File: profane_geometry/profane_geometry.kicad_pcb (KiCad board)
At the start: 4 copper layers, 71.1 x 53.3 mm, 105 parts, among them J1 Conn_01x12, J2 Conn_01x12, Q1 MMBF4416A, U1 LM1117-3.3, U2 TL074, U3 TL074, U4 TL074, U5 TL074, U6 TL072, U7 MCP6002-xSN, U8 MCP4728

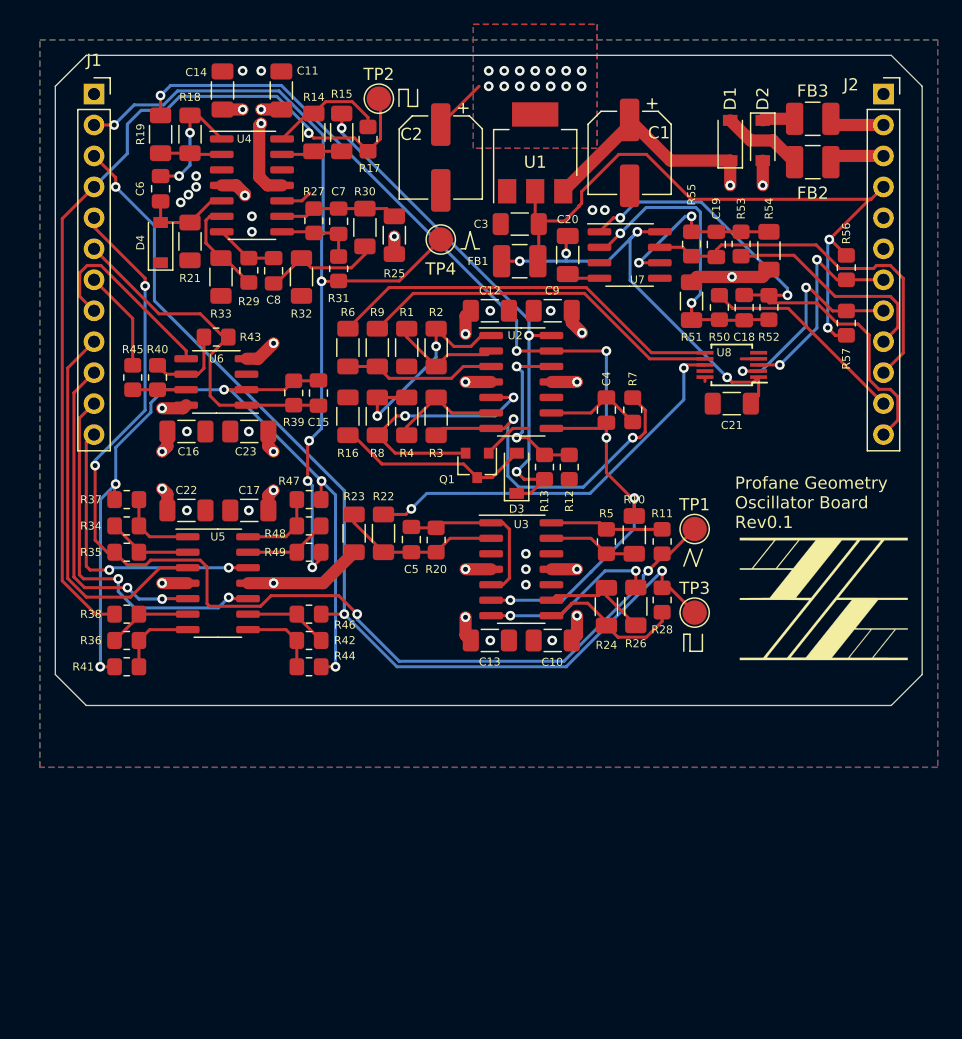
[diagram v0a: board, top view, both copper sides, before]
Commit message: update .gitignore, current kicad project
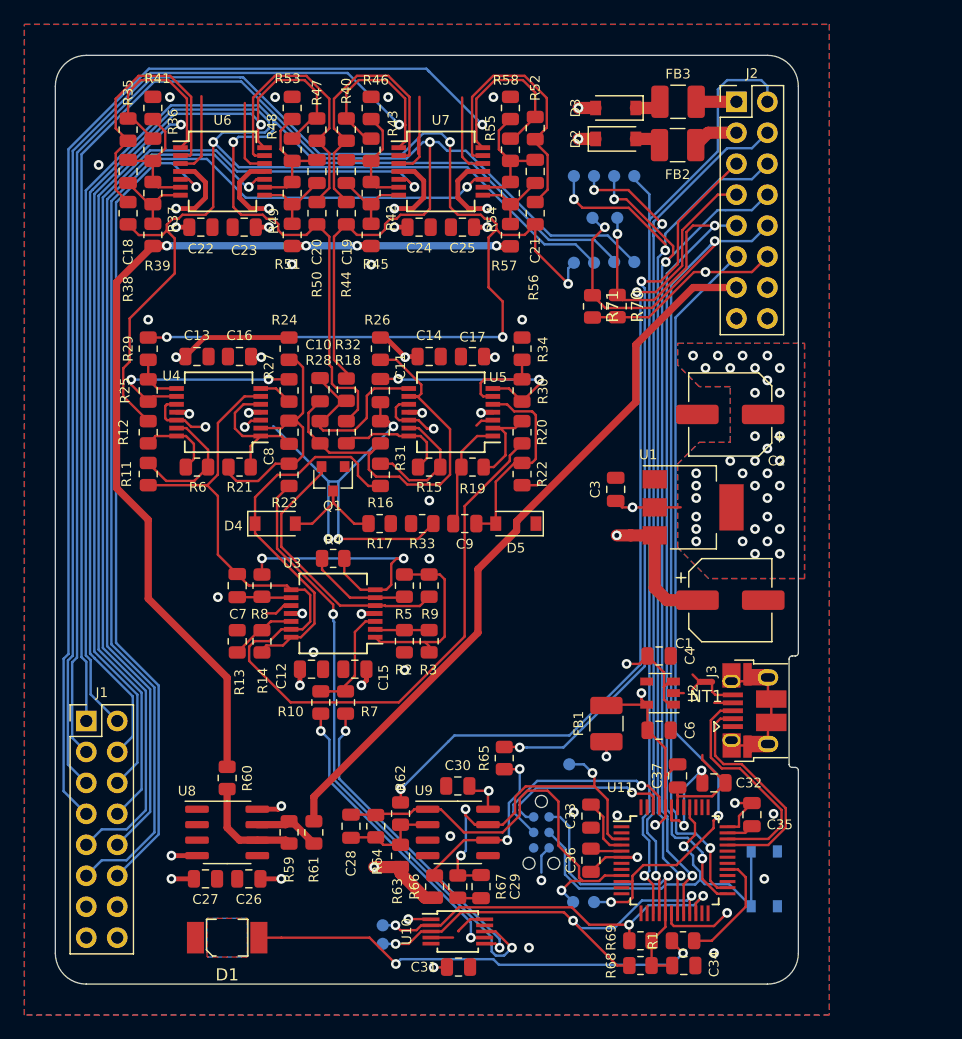
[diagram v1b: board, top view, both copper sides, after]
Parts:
- removed C5: 2.2nF, Capacitor_SMD:C_0805_2012Metric_Pad1.18x1.45mm_HandSolder
- removed REF**: OSHW-Symbol_6.7x6mm_SilkScreen, profane_geometry:OSHW-Symbol_6.7x6mm_SilkScreen
- removed Ref**: Val**, profane_geometry:zzzzzzzz_back_soldermask
- removed Ref**: Val**, profane_geometry:zzzzzzzz_new_front_soldermask
- added C24: 0.1uF, Capacitor_SMD:C_0805_2012Metric, F.Cu at (146.7, 59.8)
- added C25: 0.1uF, Capacitor_SMD:C_0805_2012Metric, F.Cu at (150.2, 59.8)
- added C26: 0.1uF, Capacitor_SMD:C_0805_2012Metric, F.Cu at (132.7, 113.3)
- added C27: 0.1uF, Capacitor_SMD:C_0805_2012Metric, F.Cu at (129.2, 113.3)
- added C28: 4.7nF, Capacitor_SMD:C_0805_2012Metric, F.Cu at (141.1, 109.0)
- added C29: 2.2nF, Capacitor_SMD:C_0805_2012Metric, F.Cu at (151.8, 113.9)
- added C30: 0.1uF, Capacitor_SMD:C_0805_2012Metric, F.Cu at (149.9, 105.7)
- added C31: 0.1uF, Capacitor_SMD:C_0805_2012Metric, F.Cu at (149.9, 120.5)
- added C32: 1uF, Capacitor_SMD:C_0805_2012Metric, F.Cu at (170.9, 105.4)
- added C33: 0.1uF, Capacitor_SMD:C_0805_2012Metric, F.Cu at (160.8, 108.1)
- added C34: 0.1uF, Capacitor_SMD:C_0805_2012Metric, F.Cu at (168.4, 120.4)
- added C35: 0.1uF, Capacitor_SMD:C_0805_2012Metric, F.Cu at (174.0, 108.0)
- added C36: 0.1uF, Capacitor_SMD:C_0805_2012Metric, F.Cu at (160.8, 111.8)
- added C37: 0.1uF, Capacitor_SMD:C_0805_2012Metric, F.Cu at (167.9, 104.8)
- added D5: 1N5819, Diode_SMD:D_SOD-123, F.Cu at (154.6, 84.1)
- added J3: USB_B_Micro, Connector_USB:USB_Micro-B_Amphenol_10103594-0001LF_Horizontal, F.Cu at (174.2, 99.5)
- added J4: TagConect SWD, Connector:Tag-Connect_TC2030-IDC-NL_2x03_P1.27mm_Vertical, B.Cu at (156.7, 109.5)
- added NT1: GND_Net_Tie, NetTie:NetTie-2_SMD_Pad0.5mm, F.Cu at (170.2, 97.1)
- added R58: 22k, Resistor_SMD:R_0805_2012Metric, F.Cu at (154.2, 50.0)
- added R59: 10k, Resistor_SMD:R_0805_2012Metric, F.Cu at (136.0, 109.5)
- added R60: 10k, Resistor_SMD:R_0805_2012Metric, F.Cu at (130.9, 105.0)
- added R61: 1k, Resistor_SMD:R_0805_2012Metric, F.Cu at (138.0, 109.5)
- added R62: 100k, Resistor_SMD:R_0805_2012Metric, F.Cu at (145.2, 107.9)
- added R63: 240k, Resistor_SMD:R_0805_2012Metric, F.Cu at (145.2, 111.4)
- added R64: 64.9k, Resistor_SMD:R_0805_2012Metric, F.Cu at (143.1, 109.0)
- added R65: 100k, Resistor_SMD:R_0805_2012Metric, F.Cu at (153.7, 103.4)
- added R66: 240k, Resistor_SMD:R_0805_2012Metric, F.Cu at (148.0, 113.9)
- added R67: 56k, Resistor_SMD:R_0805_2012Metric, F.Cu at (149.9, 113.9)
- added R68: 4.7k, Resistor_SMD:R_0805_2012Metric, F.Cu at (164.8, 120.4)
- added R69: 4.7k, Resistor_SMD:R_0805_2012Metric, F.Cu at (164.8, 118.4)
- added R70: 4.7k, Resistor_SMD:R_0805_2012Metric, F.Cu at (162.9, 66.3)
- added R71: 4.7k, Resistor_SMD:R_0805_2012Metric, F.Cu at (160.9, 66.3)
- added SW1: RESET_SW, zzzzzzzz:SPST_TL3365AF180QG_SMD, B.Cu at (175.0, 113.3)
- added TP10: PSL, TestPoint:TestPoint_Pad_D1.0mm, B.Cu at (159.4, 55.6)
- added TP11: NSL, TestPoint:TestPoint_Pad_D1.0mm, B.Cu at (162.7, 55.6)
- added TP12: D_SDA, TestPoint:TestPoint_Pad_D1.0mm, B.Cu at (143.7, 118.6)
- added TP13: D_SCL, TestPoint:TestPoint_Pad_D1.0mm, B.Cu at (143.7, 117.1)
- added TP14: L_SDA, TestPoint:TestPoint_Pad_D1.0mm, B.Cu at (162.9, 59.1)
- added TP15: L_SCL, TestPoint:TestPoint_Pad_D1.0mm, B.Cu at (160.9, 59.1)
- added TP5: V/OCT, TestPoint:TestPoint_Pad_D1.0mm, B.Cu at (159.0, 103.9)
- added TP6: PWM, TestPoint:TestPoint_Pad_D1.0mm, B.Cu at (159.3, 115.2)
- added TP7: POT, TestPoint:TestPoint_Pad_D1.0mm, B.Cu at (161.0, 115.2)
- added TP8: TSL, TestPoint:TestPoint_Pad_D1.0mm, B.Cu at (164.3, 55.6)
- added TP9: SSL, TestPoint:TestPoint_Pad_D1.0mm, B.Cu at (161.0, 55.6)
- added U10: MCP4728, Package_SO:MSOP-10_3x3mm_P0.5mm, F.Cu at (149.9, 117.6)
- added U11: ATSAMD21G18A-AUT, Package_QFP:TQFP-48_7x7mm_P0.5mm, F.Cu at (167.6, 111.8)
- added U9: MCP6002-xSN, Package_SO:SOIC-8_3.9x4.9mm_P1.27mm, F.Cu at (149.9, 109.5)
- C10: value 0.1uF -> 22pF; footprint Capacitor_SMD:C_1206_3216Metric_Pad1.33x1.80mm_HandSolder -> Capacitor_SMD:C_0805_2012Metric
- C11: value 0.1uF -> 4.7uF; footprint Capacitor_SMD:C_1206_3216Metric_Pad1.33x1.80mm_HandSolder -> Capacitor_SMD:C_0805_2012Metric
- C12, C13, C14, C16, C17, C22, C23, C3: footprint Capacitor_SMD:C_1206_3216Metric_Pad1.33x1.80mm_HandSolder -> Capacitor_SMD:C_0805_2012Metric
- C15: value 8.2pF -> 0.1uF; footprint Capacitor_SMD:C_0805_2012Metric_Pad1.18x1.45mm_HandSolder -> Capacitor_SMD:C_0805_2012Metric
- C18: value 4.7nF -> 47pF; footprint Capacitor_SMD:C_0805_2012Metric_Pad1.18x1.45mm_HandSolder -> Capacitor_SMD:C_0805_2012Metric
- C19: value 2.2nF -> 47pF; footprint Capacitor_SMD:C_0805_2012Metric_Pad1.18x1.45mm_HandSolder -> Capacitor_SMD:C_0805_2012Metric
- C20, C21: value 0.1uF -> 47pF; footprint Capacitor_SMD:C_1206_3216Metric_Pad1.33x1.80mm_HandSolder -> Capacitor_SMD:C_0805_2012Metric
- C4: value 47nF -> 1uF; footprint Capacitor_SMD:C_0805_2012Metric_Pad1.18x1.45mm_HandSolder -> Capacitor_SMD:C_0805_2012Metric
- C6: value 10uF -> 1uF; footprint Capacitor_SMD:C_0805_2012Metric_Pad1.18x1.45mm_HandSolder -> Capacitor_SMD:C_0805_2012Metric
- C7: value 22pF -> 47nF; footprint Capacitor_SMD:C_0805_2012Metric_Pad1.18x1.45mm_HandSolder -> Capacitor_SMD:C_0805_2012Metric
- C8: value 10uF -> 2.2nF; footprint Capacitor_SMD:C_0805_2012Metric_Pad1.18x1.45mm_HandSolder -> Capacitor_SMD:C_0805_2012Metric
- C9: value 0.1uF -> 1uF; footprint Capacitor_SMD:C_1206_3216Metric_Pad1.33x1.80mm_HandSolder -> Capacitor_SMD:C_0805_2012Metric
- D1: value 1N5819 -> PWR; footprint Diode_SMD:D_SOD-123 -> zzzzzzzz:SunLED-Rev-2-PLCC-SeeThru
- J1, J2: value Conn_01x12 -> Conn_02x08_Odd_Even; footprint Connector_PinSocket_2.54mm:PinSocket_1x12_P2.54mm_Vertical -> Connector_PinHeader_2.54mm:PinHeader_2x08_P2.54mm_Vertical
- R1: value 10k -> 330R; footprint Resistor_SMD:R_1206_3216Metric_Pad1.30x1.75mm_HandSolder -> Resistor_SMD:R_0805_2012Metric
- R10: value 10k -> 1M; footprint Resistor_SMD:R_1206_3216Metric_Pad1.30x1.75mm_HandSolder -> Resistor_SMD:R_0805_2012Metric
- R11, R17, R31, R45, R7: value 1k -> 10k; footprint Resistor_SMD:R_0805_2012Metric_Pad1.20x1.40mm_HandSolder -> Resistor_SMD:R_0805_2012Metric
- R12: value 7.15k -> 1k; footprint Resistor_SMD:R_0805_2012Metric_Pad1.20x1.40mm_HandSolder -> Resistor_SMD:R_0805_2012Metric
- R13: value 2.87k -> 7.15k; footprint Resistor_SMD:R_0805_2012Metric_Pad1.20x1.40mm_HandSolder -> Resistor_SMD:R_0805_2012Metric
- R14: value 4.12k -> 2.87k; footprint Resistor_SMD:R_1206_3216Metric_Pad1.30x1.75mm_HandSolder -> Resistor_SMD:R_0805_2012Metric
- R15: value 10k -> 4.12k; footprint Resistor_SMD:R_1206_3216Metric_Pad1.30x1.75mm_HandSolder -> Resistor_SMD:R_0805_2012Metric
- R16, R2, R3, R4: footprint Resistor_SMD:R_1206_3216Metric_Pad1.30x1.75mm_HandSolder -> Resistor_SMD:R_0805_2012Metric
- R18: value 3.57k -> 1k; footprint Resistor_SMD:R_1206_3216Metric_Pad1.30x1.75mm_HandSolder -> Resistor_SMD:R_0805_2012Metric
- R19: value 10k -> 3.57k; footprint Resistor_SMD:R_1206_3216Metric_Pad1.30x1.75mm_HandSolder -> Resistor_SMD:R_0805_2012Metric
- R20: value 169k -> 10k; footprint Resistor_SMD:R_0805_2012Metric_Pad1.20x1.40mm_HandSolder -> Resistor_SMD:R_0805_2012Metric
- R21: value 47k -> 169k; footprint Resistor_SMD:R_1206_3216Metric_Pad1.30x1.75mm_HandSolder -> Resistor_SMD:R_0805_2012Metric
- R22: value 33k -> 47k; footprint Resistor_SMD:R_1206_3216Metric_Pad1.30x1.75mm_HandSolder -> Resistor_SMD:R_0805_2012Metric
- R23: value 240k -> 49.9k; footprint Resistor_SMD:R_1206_3216Metric_Pad1.30x1.75mm_HandSolder -> Resistor_SMD:R_0805_2012Metric
- R24: value 10k -> 240k; footprint Resistor_SMD:R_1206_3216Metric_Pad1.30x1.75mm_HandSolder -> Resistor_SMD:R_0805_2012Metric
- R25: value 47k -> 10k; footprint Resistor_SMD:R_1206_3216Metric_Pad1.30x1.75mm_HandSolder -> Resistor_SMD:R_0805_2012Metric
- R26: value 22k -> 47k; footprint Resistor_SMD:R_1206_3216Metric_Pad1.30x1.75mm_HandSolder -> Resistor_SMD:R_0805_2012Metric
- R27: value 8.25k -> 22k; footprint Resistor_SMD:R_0805_2012Metric_Pad1.20x1.40mm_HandSolder -> Resistor_SMD:R_0805_2012Metric
- R28: value 1k -> 8.25k; footprint Resistor_SMD:R_0805_2012Metric_Pad1.20x1.40mm_HandSolder -> Resistor_SMD:R_0805_2012Metric
- R29: value 30.1k -> 1k; footprint Resistor_SMD:R_0805_2012Metric_Pad1.20x1.40mm_HandSolder -> Resistor_SMD:R_0805_2012Metric
- R30: value 10k -> 30.1k; footprint Resistor_SMD:R_1206_3216Metric_Pad1.30x1.75mm_HandSolder -> Resistor_SMD:R_0805_2012Metric
- R32: value 47k -> 1k; footprint Resistor_SMD:R_1206_3216Metric_Pad1.30x1.75mm_HandSolder -> Resistor_SMD:R_0805_2012Metric
- R33: value 10k -> 100k; footprint Resistor_SMD:R_1206_3216Metric_Pad1.30x1.75mm_HandSolder -> Resistor_SMD:R_0805_2012Metric
- R34, R35, R40: value 20k -> 10k; footprint Resistor_SMD:R_0805_2012Metric_Pad1.20x1.40mm_HandSolder -> Resistor_SMD:R_0805_2012Metric
- R36, R43, R48: value 20k -> 2.2M; footprint Resistor_SMD:R_0805_2012Metric_Pad1.20x1.40mm_HandSolder -> Resistor_SMD:R_0805_2012Metric
- R37: value 100k -> 47k; footprint Resistor_SMD:R_0805_2012Metric_Pad1.20x1.40mm_HandSolder -> Resistor_SMD:R_0805_2012Metric
- R38: value 20k -> 30.1k; footprint Resistor_SMD:R_0805_2012Metric_Pad1.20x1.40mm_HandSolder -> Resistor_SMD:R_0805_2012Metric
- R39, R47: value 100k -> 10k; footprint Resistor_SMD:R_0805_2012Metric_Pad1.20x1.40mm_HandSolder -> Resistor_SMD:R_0805_2012Metric
- R41, R53: value 100k -> 22k; footprint Resistor_SMD:R_0805_2012Metric_Pad1.20x1.40mm_HandSolder -> Resistor_SMD:R_0805_2012Metric
- R42, R49: value 20k -> 47k; footprint Resistor_SMD:R_0805_2012Metric_Pad1.20x1.40mm_HandSolder -> Resistor_SMD:R_0805_2012Metric
- R44, R50: value 100k -> 30.1k; footprint Resistor_SMD:R_0805_2012Metric_Pad1.20x1.40mm_HandSolder -> Resistor_SMD:R_0805_2012Metric
- R46: value 20k -> 22k; footprint Resistor_SMD:R_0805_2012Metric_Pad1.20x1.40mm_HandSolder -> Resistor_SMD:R_0805_2012Metric
- R5: value 5.9k -> 10k; footprint Resistor_SMD:R_0805_2012Metric_Pad1.20x1.40mm_HandSolder -> Resistor_SMD:R_0805_2012Metric
- R51: value 240k -> 10k; footprint Resistor_SMD:R_1206_3216Metric_Pad1.30x1.75mm_HandSolder -> Resistor_SMD:R_0805_2012Metric
- R52: value 64.9k -> 10k; footprint Resistor_SMD:R_0805_2012Metric_Pad1.20x1.40mm_HandSolder -> Resistor_SMD:R_0805_2012Metric
- R54: value 240k -> 47k; footprint Resistor_SMD:R_1206_3216Metric_Pad1.30x1.75mm_HandSolder -> Resistor_SMD:R_0805_2012Metric
- R55: value 56k -> 2.2M; footprint Resistor_SMD:R_0805_2012Metric_Pad1.20x1.40mm_HandSolder -> Resistor_SMD:R_0805_2012Metric
- R56: value 4.7k -> 30.1k; footprint Resistor_SMD:R_0805_2012Metric_Pad1.20x1.40mm_HandSolder -> Resistor_SMD:R_0805_2012Metric
- R57: value 4.7k -> 10k; footprint Resistor_SMD:R_0805_2012Metric_Pad1.20x1.40mm_HandSolder -> Resistor_SMD:R_0805_2012Metric
- R6: value 10k -> 5.6k; footprint Resistor_SMD:R_1206_3216Metric_Pad1.30x1.75mm_HandSolder -> Resistor_SMD:R_0805_2012Metric
- R8: value 10k -> 1k; footprint Resistor_SMD:R_1206_3216Metric_Pad1.30x1.75mm_HandSolder -> Resistor_SMD:R_0805_2012Metric
- R9: value 1M -> 10k; footprint Resistor_SMD:R_1206_3216Metric_Pad1.30x1.75mm_HandSolder -> Resistor_SMD:R_0805_2012Metric
- TP1, TP2, TP3, TP4: footprint TestPoint:TestPoint_Pad_D2.0mm -> TestPoint:TestPoint_Pad_D1.0mm; moved to B.Cu
- U1: value LM1117-3.3 -> LM1117-5
- U2: value TL074 -> AP2112K-3.3; footprint Package_SO:SOIC-14_3.9x8.7mm_P1.27mm -> Package_TO_SOT_SMD:SOT-23-5
- U3, U4, U5: footprint Package_SO:SOIC-14_3.9x8.7mm_P1.27mm -> Package_SO:SSOP-14_5.3x6.2mm_P0.65mm
- U6: value TL072 -> TL074; footprint Package_SO:SOIC-8_3.9x4.9mm_P1.27mm -> Package_SO:SSOP-14_5.3x6.2mm_P0.65mm
- U7: value MCP6002-xSN -> TL074; footprint Package_SO:SOIC-8_3.9x4.9mm_P1.27mm -> Package_SO:SSOP-14_5.3x6.2mm_P0.65mm
- U8: value MCP4728 -> TL072; footprint Package_SO:MSOP-10_3x3mm_P0.5mm -> Package_SO:SOIC-8_3.9x4.9mm_P1.27mm
- moved D1 77.3 mm to (130.9, 118.1), turned to 0 degrees
- moved C6 60.4 mm to (166.4, 101.1), turned to 0 degrees
- moved U8 56.4 mm to (130.9, 109.5), turned to 0 degrees
- moved R1 53.7 mm to (168.3, 118.4), turned to 180 degrees
- moved C18 51.8 mm to (122.8, 55.2), turned to 90 degrees
- moved J1 51.4 mm to (119.4, 100.3)
- moved R41 45.9 mm to (124.8, 50.0), turned to 270 degrees
- moved R11 42.5 mm to (124.5, 80.1), turned to 270 degrees
- moved R14 42.0 mm to (133.8, 93.8), turned to 90 degrees
- moved R46 41.8 mm to (142.7, 50.0), turned to 270 degrees
- moved R36 40.3 mm to (124.8, 53.5), turned to 90 degrees
- moved FB1 38.6 mm to (162.1, 100.5), turned to 90 degrees
- moved R53 38.5 mm to (136.3, 50.0)
- moved C1 37.6 mm to (172.2, 90.4), turned to 0 degrees
- moved R19 37.4 mm to (151.1, 79.5), turned to 0 degrees
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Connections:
- C10 pad 1: GND -> Net-(C10-Pad1)
- C10 pad 2: -12V -> Net-(C10-Pad2)
- C11 pad 1: GND -> Net-(C11-Pad1)
- C11 pad 2: -12V -> Net-(C11-Pad2)
- C12 pad 1: +12V -> GND
- C12 pad 2: GND -> -12V
- C13 pad 1: +12V -> GND
- C13 pad 2: GND -> -12V
- C14 pad 1: +12V -> GND
- C14 pad 2: GND -> -12V
- C15 pad 1: /mix-pre -> +12V
- C15 pad 2: Net-(C15-Pad2) -> GND
- C17 pad 1: GND -> +12V
- C17 pad 2: -12V -> GND
- C18 pad 1: /pulse-scaled -> Net-(C18-Pad1)
- C19 pad 1: /v_oct-scaled -> Net-(C19-Pad1)
- C2 pad 1: +3V3 -> +5V
- C20 pad 1: GND -> Net-(C20-Pad1)
- C20 pad 2: +3.3VA -> Net-(C20-Pad2)
- C21 pad 1: GND -> Net-(C21-Pad1)
- C21 pad 2: +3.3VA -> Net-(C21-Pad2)
- C3 pad 1: +3V3 -> +5V
- C4 pad 1: /Geometry Core/tri-pre -> +5V
- C4 pad 2: Net-(C4-Pad2) -> GND
- C6 pad 1: Net-(C6-Pad1) -> +3V3
- C6 pad 2: Net-(C6-Pad2) -> GND
- C7 pad 1: Net-(C7-Pad1) -> /Geometry Core/tri-pre
- C9 pad 1: GND -> Net-(C9-Pad1)
- C9 pad 2: -12V -> Net-(C9-Pad2)
- D1 pad 1: +12V -> GND
- D2 pad 1: Net-(D2-Pad1) -> +12V
- D2 pad 2: -12V -> Net-(D2-Pad2)
- D3 pad 1: /Geometry Core/square-pre -> Net-(D3-Pad1)
- D3 pad 2: Net-(D3-Pad2) -> -12V
- D4 pad 1: GND -> /Geometry Core/square-pre
- D4 pad 2: Net-(C6-Pad1) -> Net-(D4-Pad2)
- FB2 pad 1: Net-(D1-Pad2) -> Net-(D2-Pad2)
- FB3 pad 1: Net-(D2-Pad1) -> Net-(D3-Pad1)
- J1 pad 1: GND -> /notch-out
- J1 pad 10: /square-att-in -> /square-mix-in
- J1 pad 11: /pulse-att-in -> /pulse-mix-in
- J1 pad 12: /notch-att-in -> /tri-mix-in
- J1 pad 2: /notch-out -> /square-out
- J1 pad 4: /square-out -> /tri-out
- J1 pad 5: /tri-out -> /notch-pre-out
- J1 pad 6: /mix-pre -> /square-pre-out
- J1 pad 7: /mix-out -> /pulse-pre-out
- J1 pad 8: /mix-att-in -> /tri-pre-out
- J1 pad 9: /tri-att-in -> /notch-mix-in
- J2 pad 1: GND -> /-12v-rack
- J2 pad 10: /v_oct-scaled -> /rgb-scl
- J2 pad 11: /pulse-cv -> /pulse-pot-in
- J2 pad 12: /pulse-scaled -> +3V3
- J2 pad 2: /-12v-rack -> /tri-slider-led
- J2 pad 4: +3V3 -> /square-slider-led
- J2 pad 5: Net-(J2-Pad5) -> /v_oct-cv
- J2 pad 6: Net-(J2-Pad6) -> /pulse-slider-led
- J2 pad 7: /SERCOM4[0] -> /pulse-cv
- J2 pad 8: /SERCOM4[1] -> /notch-slider-led
- J2 pad 9: /v_oct-cv -> /rgb-sda
- Q1 pad 3: Net-(D3-Pad2) -> Net-(D4-Pad2)
- R1 pad 1: Net-(R1-Pad1) -> /MCU/TCC0_WO[6]
- R1 pad 2: GND -> Net-(D1-Pad2)
- R10 pad 2: /Geometry Core/tri-pre -> /dac-fine-cv
- R11 pad 1: /tri-out -> Net-(R11-Pad1)
- R11 pad 2: Net-(R11-Pad2) -> /Geometry Core/tri-pre
- R12 pad 1: Net-(R12-Pad1) -> /tri-out
- R12 pad 2: GND -> Net-(R12-Pad2)
- R13 pad 1: /Geometry Core/square-pre -> Net-(R13-Pad1)
- R13 pad 2: Net-(R12-Pad1) -> GND
- R14 pad 1: Net-(R14-Pad1) -> /Geometry Core/square-pre
- R14 pad 2: Net-(R14-Pad2) -> Net-(R13-Pad1)
- R15 pad 1: Net-(R14-Pad2) -> Net-(R15-Pad1)
- R15 pad 2: /Geometry Core/square-pre -> Net-(R15-Pad2)
- R16 pad 1: GND -> Net-(R15-Pad2)
- R16 pad 2: Net-(D3-Pad2) -> /Geometry Core/square-pre
- R17 pad 1: /square-out -> GND
- R17 pad 2: Net-(R14-Pad1) -> Net-(D4-Pad2)
- R18 pad 1: Net-(C6-Pad2) -> /square-out
- R18 pad 2: Net-(R18-Pad2) -> Net-(R15-Pad1)
- R19 pad 1: Net-(R18-Pad2) -> Net-(C9-Pad2)
- R19 pad 2: /Geometry Core/tri-pre -> Net-(R19-Pad2)
- R2 pad 2: Net-(R1-Pad1) -> GND
- R20 pad 1: Net-(C5-Pad1) -> Net-(R19-Pad2)
- R20 pad 2: Net-(C5-Pad2) -> /Geometry Core/tri-pre
- R21 pad 1: Net-(C6-Pad1) -> Net-(C8-Pad1)
- R21 pad 2: GND -> Net-(C8-Pad2)
- R22 pad 1: Net-(C5-Pad2) -> Net-(C9-Pad1)
- R22 pad 2: /duty-cv -> GND
- R23 pad 1: Net-(C5-Pad2) -> Net-(C8-Pad2)
- R23 pad 2: -12V -> /duty-cv
- R24 pad 1: Net-(R24-Pad1) -> Net-(C8-Pad2)
- R24 pad 2: Net-(R24-Pad2) -> -12V
- R25 pad 1: Net-(C7-Pad2) -> Net-(R25-Pad1)
- R25 pad 2: -12V -> Net-(R25-Pad2)
- R26 pad 1: Net-(R24-Pad2) -> Net-(C10-Pad2)
- R26 pad 2: Net-(R26-Pad2) -> -12V
- R27 pad 1: Net-(C7-Pad1) -> Net-(R25-Pad2)
- R27 pad 2: Net-(C7-Pad2) -> Net-(R27-Pad2)
- R28 pad 1: /pulse-out -> Net-(C10-Pad1)
- R28 pad 2: Net-(R24-Pad1) -> Net-(C10-Pad2)
- R29 pad 1: Net-(C8-Pad2) -> /pulse-out
- R29 pad 2: Net-(R29-Pad2) -> Net-(R25-Pad1)
- R3 pad 2: Net-(R3-Pad2) -> Net-(R2-Pad1)
- R30 pad 1: Net-(C7-Pad2) -> Net-(C11-Pad2)
- R30 pad 2: Net-(C8-Pad1) -> Net-(R30-Pad2)
- R31 pad 1: /notch-out -> Net-(C10-Pad2)
- R31 pad 2: Net-(C7-Pad1) -> Net-(C11-Pad1)
- R32 pad 1: Net-(C8-Pad1) -> /notch-out
- R32 pad 2: GND -> Net-(C10-Pad1)
- R33 pad 1: Net-(R29-Pad2) -> Net-(C11-Pad1)
- R34 pad 1: Net-(R34-Pad1) -> Net-(R30-Pad2)
- R34 pad 2: Net-(R34-Pad2) -> GND
- R35 pad 1: Net-(R34-Pad2) -> /tri-pre-out
- R35 pad 2: /tri-out -> Net-(R35-Pad2)
- R36 pad 1: Net-(R36-Pad1) -> Net-(C18-Pad2)
- R36 pad 2: Net-(R36-Pad2) -> /tri-pre-out
- R37 pad 1: Net-(C15-Pad2) -> Net-(C18-Pad1)
- R37 pad 2: Net-(R34-Pad1) -> Net-(C18-Pad2)
- R38 pad 1: Net-(R36-Pad2) -> Net-(R35-Pad2)
- R38 pad 2: /square-out -> /tri-out
- R39 pad 1: /mix-pre -> /Mixer/notch-ch
- R39 pad 2: Net-(C15-Pad2) -> Net-(C18-Pad1)
- R4 pad 1: Net-(R3-Pad2) -> Net-(R4-Pad1)
- R4 pad 2: Net-(R2-Pad1) -> Net-(R4-Pad2)
- R40 pad 1: Net-(R40-Pad1) -> /notch-pre-out
- R41 pad 1: Net-(C15-Pad2) -> GND
- R41 pad 2: Net-(R36-Pad1) -> Net-(C18-Pad2)
- R42 pad 1: Net-(R42-Pad1) -> Net-(C19-Pad1)
- R42 pad 2: Net-(R42-Pad2) -> Net-(C19-Pad2)
- R43 pad 1: Net-(R40-Pad2) -> Net-(C19-Pad2)
- R43 pad 2: /mix-pre -> /notch-pre-out
- R44 pad 1: Net-(C15-Pad2) -> Net-(R40-Pad2)
- R44 pad 2: Net-(R42-Pad1) -> /notch-out
- R45 pad 1: /mix-out -> Net-(C19-Pad1)
- R45 pad 2: Net-(R40-Pad1) -> /Mixer/notch-ch
- R46 pad 1: Net-(R42-Pad2) -> GND
- R46 pad 2: /pulse-out -> Net-(C19-Pad2)
- R47 pad 1: Net-(C15-Pad2) -> /square-pre-out
- R48 pad 1: Net-(R47-Pad2) -> Net-(C20-Pad2)
- R48 pad 2: Net-(R48-Pad2) -> /square-pre-out
- R49 pad 1: Net-(R48-Pad2) -> Net-(C20-Pad1)
- R49 pad 2: /notch-out -> Net-(C20-Pad2)
- R5 pad 1: Net-(R11-Pad2) -> Net-(R4-Pad2)
- R5 pad 2: Net-(R10-Pad1) -> Net-(R3-Pad1)
- R50 pad 1: Net-(C18-Pad2) -> Net-(R47-Pad2)
- R50 pad 2: /pulse-cv -> /square-out
- R51 pad 1: -12V -> /Mixer/notch-ch
- R51 pad 2: Net-(C18-Pad2) -> Net-(C20-Pad1)
- R52 pad 1: Net-(C18-Pad2) -> /pulse-pre-out
- R52 pad 2: /pulse-scaled -> Net-(R52-Pad2)
- R53 pad 1: Net-(C19-Pad2) -> GND
- R53 pad 2: /v_oct-cv -> Net-(C20-Pad2)
- R54 pad 1: -12V -> Net-(C21-Pad1)
- R54 pad 2: Net-(C19-Pad2) -> Net-(C21-Pad2)
- R55 pad 1: Net-(C19-Pad2) -> Net-(C21-Pad2)
- R55 pad 2: /v_oct-scaled -> /pulse-pre-out
- R56 pad 1: +3V3 -> Net-(R52-Pad2)
- R56 pad 2: /SERCOM4[0] -> /pulse-out
- R57 pad 1: +3V3 -> Net-(C21-Pad1)
- R57 pad 2: /SERCOM4[1] -> /Mixer/notch-ch
- R6 pad 1: Net-(R6-Pad1) -> Net-(R12-Pad2)
- R6 pad 2: /dac-coarse-cv -> Net-(R11-Pad1)
- R7 pad 1: Net-(C4-Pad2) -> Net-(R10-Pad1)
- R7 pad 2: Net-(R3-Pad1) -> /dac-coarse-cv
- R8 pad 1: Net-(Q1-Pad2) -> Net-(C7-Pad2)
- R8 pad 2: Net-(R2-Pad1) -> Net-(R4-Pad1)
- R9 pad 1: Net-(R6-Pad1) -> Net-(Q1-Pad2)
- R9 pad 2: /dac-fine-cv -> Net-(R3-Pad1)
- U1 pad 2: +3V3 -> +5V
- U2 pad 1: Net-(R2-Pad1) -> +5V
- U2 pad 2: Net-(R1-Pad1) -> GND
- U2 pad 3: Net-(R6-Pad1) -> +5V
- U2 pad 4: +12V -> Net-(U2-Pad4)
- U2 pad 5: Net-(Q1-Pad2) -> +3V3
- U3 pad 1: Net-(C5-Pad1) -> Net-(R3-Pad1)
- U3 pad 12: GND -> Net-(R13-Pad1)
- U3 pad 13: Net-(R10-Pad1) -> /Geometry Core/tri-pre
- U3 pad 14: Net-(R11-Pad2) -> /Geometry Core/square-pre
- U3 pad 2: Net-(C5-Pad2) -> Net-(R2-Pad1)
- U3 pad 3: GND -> Net-(R10-Pad1)
- U3 pad 5: Net-(C5-Pad1) -> Net-(Q1-Pad2)
- U3 pad 6: /Geometry Core/tri-pre -> Net-(R4-Pad2)
- U3 pad 7: Net-(R26-Pad2) -> Net-(R4-Pad1)
- U3 pad 8: Net-(R24-Pad1) -> /Geometry Core/tri-pre
- U3 pad 9: Net-(R24-Pad2) -> Net-(C7-Pad2)
- U4 pad 1: Net-(C6-Pad2) -> Net-(C8-Pad1)
- U4 pad 13: Net-(R14-Pad2) -> Net-(R11-Pad1)
- U4 pad 14: Net-(R14-Pad1) -> Net-(R12-Pad2)
- U4 pad 2: Net-(R18-Pad2) -> Net-(C8-Pad2)
- U4 pad 5: Net-(C6-Pad1) -> Net-(C8-Pad1)
- U4 pad 6: Net-(R29-Pad2) -> /Geometry Core/tri-pre
- U4 pad 7: Net-(C8-Pad2) -> Net-(R27-Pad2)
- U4 pad 8: Net-(C7-Pad1) -> Net-(R25-Pad1)
- U4 pad 9: Net-(C7-Pad2) -> Net-(R25-Pad2)
- U5 pad 1: Net-(R34-Pad1) -> Net-(C9-Pad2)
- U5 pad 10: /pulse-att-in -> GND
- U5 pad 12: /notch-att-in -> GND
- U5 pad 13: Net-(R48-Pad2) -> Net-(R15-Pad2)
- U5 pad 14: Net-(R47-Pad2) -> Net-(R15-Pad1)
- U5 pad 2: Net-(R34-Pad2) -> Net-(R19-Pad2)
- U5 pad 3: /tri-att-in -> GND
- U5 pad 5: /square-att-in -> Net-(C9-Pad1)
- U5 pad 6: Net-(R36-Pad2) -> Net-(R30-Pad2)
- U5 pad 7: Net-(R36-Pad1) -> Net-(C11-Pad2)
- U5 pad 8: Net-(R42-Pad1) -> Net-(C10-Pad1)
- U5 pad 9: Net-(R42-Pad2) -> Net-(C10-Pad2)
- U6 pad 1: /mix-pre -> /tri-pre-out
- U6 pad 2: Net-(C15-Pad2) -> Net-(R35-Pad2)
- U6 pad 4: -12V -> +12V
- U6 pad 5: /mix-att-in -> /tri-mix-in
- U6 pad 6: Net-(R40-Pad2) -> Net-(C18-Pad2)
- U6 pad 7: Net-(R40-Pad1) -> Net-(C18-Pad1)
- U6 pad 8: +12V -> Net-(C20-Pad1)
- U7 pad 1: /pulse-scaled -> /notch-pre-out
- U7 pad 2: Net-(C18-Pad2) -> Net-(R40-Pad2)
- U7 pad 4: GND -> +12V
- U7 pad 5: GND -> /notch-mix-in
- U7 pad 7: /v_oct-scaled -> Net-(C19-Pad1)
- U7 pad 8: +3.3VA -> Net-(C21-Pad1)
- U8 pad 1: +3.3VA -> (no net)
- U8 pad 2: /SERCOM4[1] -> (no net)
- U8 pad 3: /SERCOM4[0] -> (no net)
- U8 pad 4: GND -> -12V
- U8 pad 5: Net-(U8-Pad5) -> GND
- U8 pad 6: /dac-coarse-cv -> Net-(R59-Pad2)
- U8 pad 7: /dac-fine-cv -> Net-(R59-Pad1)
- U8 pad 8: /duty-cv -> +12V
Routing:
- net /pulse-pre-out: track 0.00 -> 109.9 mm, vias 0 -> 1
- net /notch-pre-out: track 0.00 -> 99.8 mm, vias 0 -> 1
- net /pulse-mix-in: track 0.00 -> 94.2 mm, vias 0 -> 1
- net /notch-mix-in: track 0.00 -> 87.7 mm, vias 0 -> 1
- net /rgb-scl: track 0.00 -> 83.5 mm, vias 0 -> 3
- net /square-pre-out: track 0.00 -> 82.6 mm, vias 0 -> 1
- net /tri-slider-led: track 0.00 -> 81.1 mm, vias 0 -> 1
- net /rgb-sda: track 0.00 -> 80.1 mm, vias 0 -> 3
- net /pulse-slider-led: track 0.00 -> 79.7 mm, vias 0 -> 3
- net /Mixer/notch-ch: track 0.00 -> 79.4 mm, vias 0 -> 4
- net /square-slider-led: track 0.00 -> 79.1 mm, vias 0 -> 3
- net /tri-pre-out: track 0.00 -> 77.6 mm, vias 0 -> 1
- net /notch-slider-led: track 0.00 -> 75.4 mm, vias 0 -> 3
- net /square-mix-in: track 0.00 -> 71.3 mm, vias 0 -> 1
- net Net-(C15-Pad2): track 69.9 -> 0.00 mm, vias 5 -> 0
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- added copper zone on B.Cu, net (none)
- added copper zone on F.Cu, net (none)
- added copper zone on B.Cu, net +5V
- added copper zone on F.Cu, net +5V
- removed copper zone on B.Cu, net +3V3
- removed copper zone on F.Cu, net +3V3
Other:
- board size 71.1 x 53.3 mm -> 61 x 76.2 mm
- net class 12V or -12V: clearance 0.4 -> 0.15; trace_width 1 -> 0.4
- net class Default: clearance 0.2 -> 0.15; trace_width 0.25 -> 0.2
- net class Mix Bus added: clearance 0.15, trace_width 0.6, via_dia 0.8, via_drill 0.4
- rule trace_clearance: 0.2 -> 0.15
- rule trace_min: 0.2 -> 0
- board text added: "DAC"
- board text added: "FP"
- board text added: "PWR"
- board text added: "UNFILL ZONES FOR PWR LED UNFILL ZONES FOR PWR LED UNFILL ZONES FOR PWR LED"
- board text removed: "14HP (2.8")"
- board text removed: "Profane Geometry Oscillator Board Rev0.1"
